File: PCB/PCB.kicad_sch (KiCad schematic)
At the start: 37 parts, among them J1 Screw_Terminal_01x02, J2 Screw_Terminal_01x02, J3 USB_C_Receptacle_USB2.0_14P, SW1 SW_Push, SW2 SW_Push, U1 MPU-6050, U2 DRV8833PWP, U3 ESP32-S3-MINI-1, U4 AP2112K-3.3

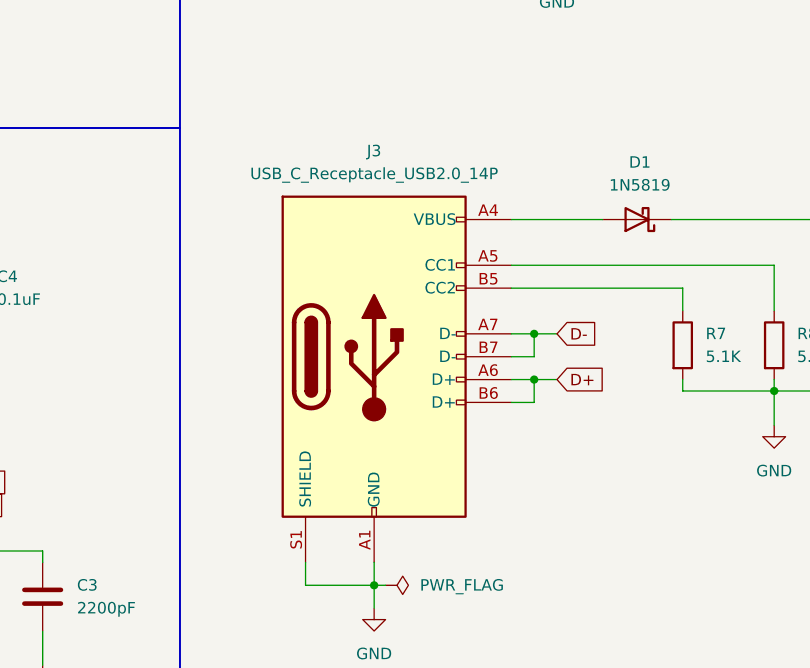
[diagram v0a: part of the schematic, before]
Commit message: PCB Progress
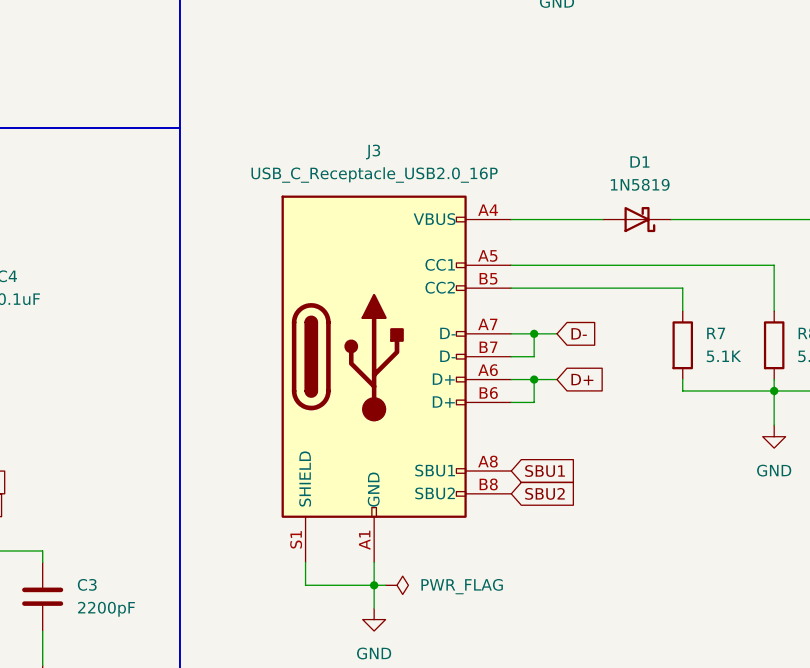
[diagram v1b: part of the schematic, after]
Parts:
- removed J3: USB_C_Receptacle_USB2.0_14P, symbol Connector:USB_C_Receptacle_USB2.0_14P
- added J3: USB_C_Receptacle_USB2.0_16P, Connector_USB:USB_C_Receptacle_G-Switch_GT-USB-7010ASV, symbol Connector:USB_C_Receptacle_USB2.0_16P
- J1: footprint Connector_Phoenix_GMSTB:PhoenixContact_GMSTBA_2,5_2-G_1x02_P7.50mm_Horizontal -> Connector_PinSocket_2.54mm:PinSocket_1x02_P2.54mm_Vertical
- J2: footprint Connector_Phoenix_GMSTB:PhoenixContact_GMSTBA_2,5_2-G_1x02_P7.50mm_Horizontal -> Connector_PinHeader_2.54mm:PinHeader_1x02_P2.54mm_Vertical
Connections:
- net D+: now also J3.A6 (D+), J3.B6 (D+)
- net D-: now also J3.A7 (D-), J3.B7 (D-)
- net GND: now also J3.A1 (GND), J3.A12 (GND), J3.B1 (GND), J3.B12 (GND), J3.S1 (SHIELD)
- net at D1.2 (A): now also J3.A4 (VBUS), J3.A9 (VBUS), J3.B4 (VBUS), J3.B9 (VBUS)
- net at R8.1: now also J3.A5 (CC1)
- net at R7.1: now also J3.B5 (CC2)
- new net SBU1: J3.A8 (SBU1)
- new net SBU2: J3.B8 (SBU2)
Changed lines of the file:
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@@
 		)
 	)
+	(global_label "SBU2"
+		(shape input)
+		(at 182.88 156.21 0)
+		(fields_autoplaced yes)
+		(effects
+			(font
+				(size 1.27 1.27)
+			)
+			(justify left)
+		)
+		(property "Intersheetrefs" "${INTERSHEET_REFS}"
+			(at 190.8847 156.21 0)
+			(effects
+				(font
+					(size 1.27 1.27)
+				)
+				(justify left)
+				(hide yes)
+			)
+		)
+	)
 	(global_label "IO46"
 		(shape input)
@@
 		)
 	)
+	(global_label "SBU1"
+		(shape input)
+		(at 182.88 153.67 0)
+		(fields_autoplaced yes)
+		(effects
+			(font
+				(size 1.27 1.27)
+			)
+			(justify left)
+		)
+		(property "Intersheetrefs" "${INTERSHEET_REFS}"
+			(at 190.8847 153.67 0)
+			(effects
+				(font
+					(size 1.27 1.27)
+				)
+				(justify left)
+				(hide yes)
+			)
+		)
+	)
 	(global_label "IO33"
 		(shape input)
@@
 			)
 		)
-		(property "Footprint" "Connector_Phoenix_GMSTB:PhoenixContact_GMSTBA_2,5_2-G_1x02_P7.50mm_Horizontal"
+		(property "Footprint" "Connector_PinHeader_2.54mm:PinHeader_1x02_P2.54mm_Vertical"
 			(at 107.95 72.39 0)
 			(effects
@@
 			)
 		)
-		(property "Footprint" "Connector_Phoenix_GMSTB:PhoenixContact_GMSTBA_2,5_2-G_1x02_P7.50mm_Horizontal"
+		(property "Footprint" "Connector_PinSocket_2.54mm:PinSocket_1x02_P2.54mm_Vertical"
 			(at 107.95 64.77 0)
 			(effects
@@
 	)
 	(symbol
+		(lib_id "Connector:USB_C_Receptacle_USB2.0_16P")
+		(at 167.64 140.97 0)
+		(unit 1)
+		(exclude_from_sim no)
+		(in_bom yes)
+		(on_board yes)
+		(dnp no)
+		(fields_autoplaced yes)
+		(property "Reference" "J3"
+			(at 167.64 118.11 0)
+			(effects
+				(font
+					(size 1.27 1.27)
+				)
+			)
+		)
+		(property "Value" "USB_C_Receptacle_USB2.0_16P"
+			(at 167.64 120.65 0)
+			(effects
+				(font
+					(size 1.27 1.27)
+				)
+			)
+		)
+		(property "Footprint" "Connector_USB:USB_C_Receptacle_G-Switch_GT-USB-7010ASV"
+			(at 171.45 140.97 0)
+			(effects
+				(font
+					(size 1.27 1.27)
+				)
+				(hide yes)
+			)
+		)
+		(property "Datasheet" "https://www.usb.org/sites/default/files/documents/usb_type-c.zip"
+			(at 171.45 140.97 0)
+			(effects
+				(font
+					(size 1.27 1.27)
+				)
+				(hide yes)
+			)
+		)
+		(property "Description" "USB 2.0-only 16P Type-C Receptacle connector"
+			(at 167.64 140.97 0)
+			(effects
+				(font
+					(size 1.27 1.27)
+				)
+				(hide yes)
+			)
+		)
+		(pin "A1"
+		)
+		(pin "B4"
+		)
+		(pin "A8"
+		)
+		(pin "A4"
+		)
+		(pin "A9"
+		)
+		(pin "A12"
+		)
+		(pin "B6"
+		)
+		(pin "B7"
+		)
+		(pin "B5"
+		)
+		(pin "A6"
+		)
+		(pin "S1"
+		)
+		(pin "A5"
+		)
+		(pin "A7"
+		)
+		(pin "B1"
+		)
+		(pin "B12"
+		)
+		(pin "B8"
+		)
+		(pin "B9"
+		)
+		(instances
+			(project ""
+				(path "/1d0c519c-16f4-4a16-b94e-0bddce7294e9"
+					(reference "J3")
+					(unit 1)
+				)
+			)
+		)
+	)
+	(symbol
 		(lib_id "Switch:SW_Push")
 		(at 270.51 152.4 270)
@@
 					(unit 1)
 				)
-			)
-		)
-	)
-	(symbol
-		(lib_id "Connector:USB_C_Receptacle_USB2.0_14P")
-		(at 167.64 140.97 0)
-		(unit 1)
-		(exclude_from_sim no)
-		(in_bom yes)
-		(on_board yes)
-		(dnp no)
-		(fields_autoplaced yes)
-		(property "Reference" "J3"
-			(at 167.64 118.11 0)
-			(effects
-				(font
-					(size 1.27 1.27)
-				)
-			)
-		)
-		(property "Value" "USB_C_Receptacle_USB2.0_14P"
-			(at 167.64 120.65 0)
-			(effects
-				(font
-					(size 1.27 1.27)
-				)
-			)
-		)
-		(property "Footprint" ""
-			(at 171.45 140.97 0)
-			(effects
-				(font
-					(size 1.27 1.27)
-				)
-				(hide yes)
-			)
-		)
-		(property "Datasheet" "https://www.usb.org/sites/default/files/documents/usb_type-c.zip"
-			(at 171.45 140.97 0)
-			(effects
-				(font
-					(size 1.27 1.27)
-				)
-				(hide yes)
-			)
-		)
-		(property "Description" "USB 2.0-only 14P Type-C Receptacle connector"
-			(at 167.64 140.97 0)
-			(effects
-				(font
-					(size 1.27 1.27)
-				)
-				(hide yes)
-			)
-		)
-		(pin "A1"
-		)
-		(pin "A5"
-		)
-		(pin "A7"
-		)
-		(pin "A9"
-		)
-		(pin "B1"
-		)
-		(pin "A4"
-		)
-		(pin "A6"
-		)
-		(pin "A12"
-		)
-		(pin "B7"
-		)
-		(pin "B4"
-		)
-		(pin "B12"
-		)
-		(pin "B5"
-		)
-		(pin "B9"
-		)
-		(pin "S1"
-		)
-		(pin "B6"
-		)
-		(instances
-			(project ""
-				(path "/1d0c519c-16f4-4a16-b94e-0bddce7294e9"
-					(reference "J3")
-					(unit 1)
-				)

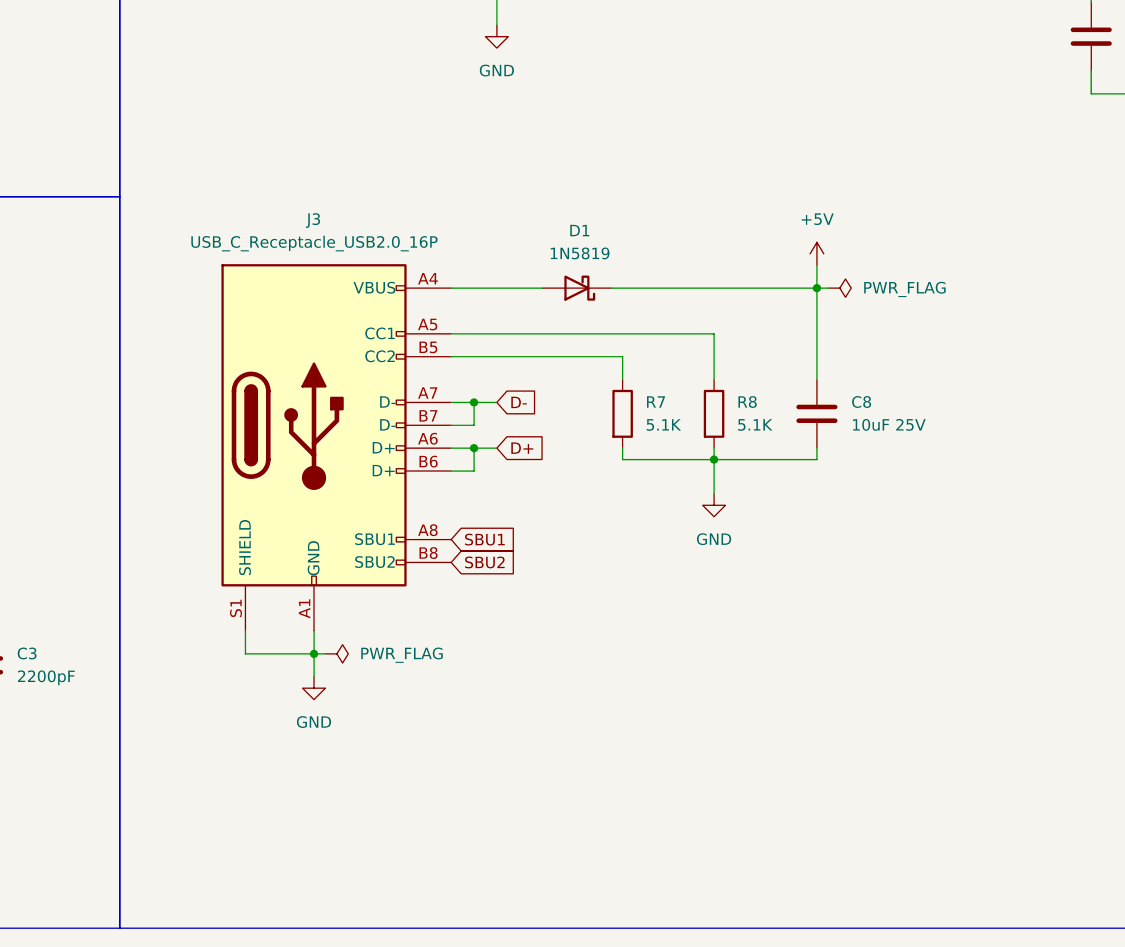
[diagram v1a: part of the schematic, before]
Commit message: Finished second PCB
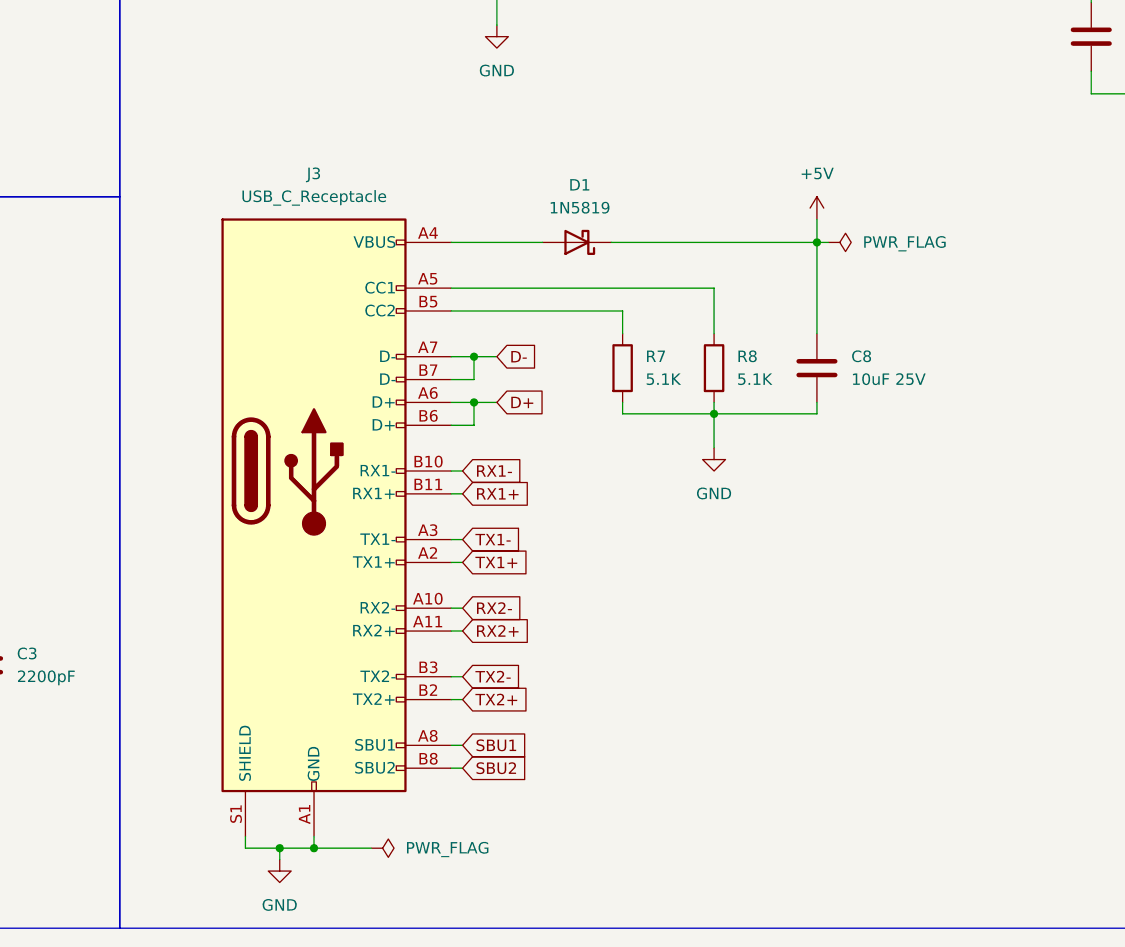
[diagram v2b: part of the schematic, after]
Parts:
- removed J3: USB_C_Receptacle_USB2.0_16P, Connector_USB:USB_C_Receptacle_G-Switch_GT-USB-7010ASV, symbol Connector:USB_C_Receptacle_USB2.0_16P
- added J3: USB_C_Receptacle, Connector_USB:USB_C_Receptacle_Amphenol_12401610E4-2A, symbol Connector:USB_C_Receptacle
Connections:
- net D+: now also J3.A6 (D+), J3.B6 (D+)
- net D-: now also J3.A7 (D-), J3.B7 (D-)
- net GND: now also J3.A1 (GND), J3.A12 (GND), J3.B1 (GND), J3.B12 (GND), J3.S1 (SHIELD)
- net SBU1: now also J3.A8 (SBU1)
- net SBU2: now also J3.B8 (SBU2)
- net at D1.2 (A): now also J3.A4 (VBUS), J3.A9 (VBUS), J3.B4 (VBUS), J3.B9 (VBUS)
- net at R8.1: now also J3.A5 (CC1)
- net at R7.1: now also J3.B5 (CC2)
- new net RX1+: J3.B11 (RX1+)
- new net RX1-: J3.B10 (RX1-)
- new net RX2+: J3.A11 (RX2+)
- new net RX2-: J3.A10 (RX2-)
- new net TX1+: J3.A2 (TX1+)
- new net TX1-: J3.A3 (TX1-)
- new net TX2+: J3.B2 (TX2+)
- new net TX2-: J3.B3 (TX2-)
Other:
- moved on the sheet: C8, D1, R7, R8
